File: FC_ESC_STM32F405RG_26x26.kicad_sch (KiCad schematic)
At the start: 211 parts, among them J1 SPI, J12 Conn_02x02_Odd_Even, J14 UART1, J15 UART3_I2C2, J16 MOTOR, J17 MOTOR, J18 MOTOR, J19 MOTOR, J2 Conn_02x04_Odd_Even, J20 USB_A, J21 ESC_PROG, J23 ESC_PROG, J24 ESC_PROG, J25 ESC_PROG, J26 LED_BUZ, J3 ST-LINK, J4 UART4, J7 RC, J8 UART6, J9 OSD, U1 EFM8BB21, U10 FD6288Q, U11 OUTLINE, U12 MPU-6000, U13 BMP280, U15 STM32F405RGTx, U16 RT9013-33GB, U2 EFM8BB21, U3 TPS54560BDDA, U4 FD6288Q, U5 FD6288Q, U6 AT7456, U7 EFM8BB21, U8 EFM8BB21, U9 FD6288Q, Y1 8MHz, Y2 8Mhz

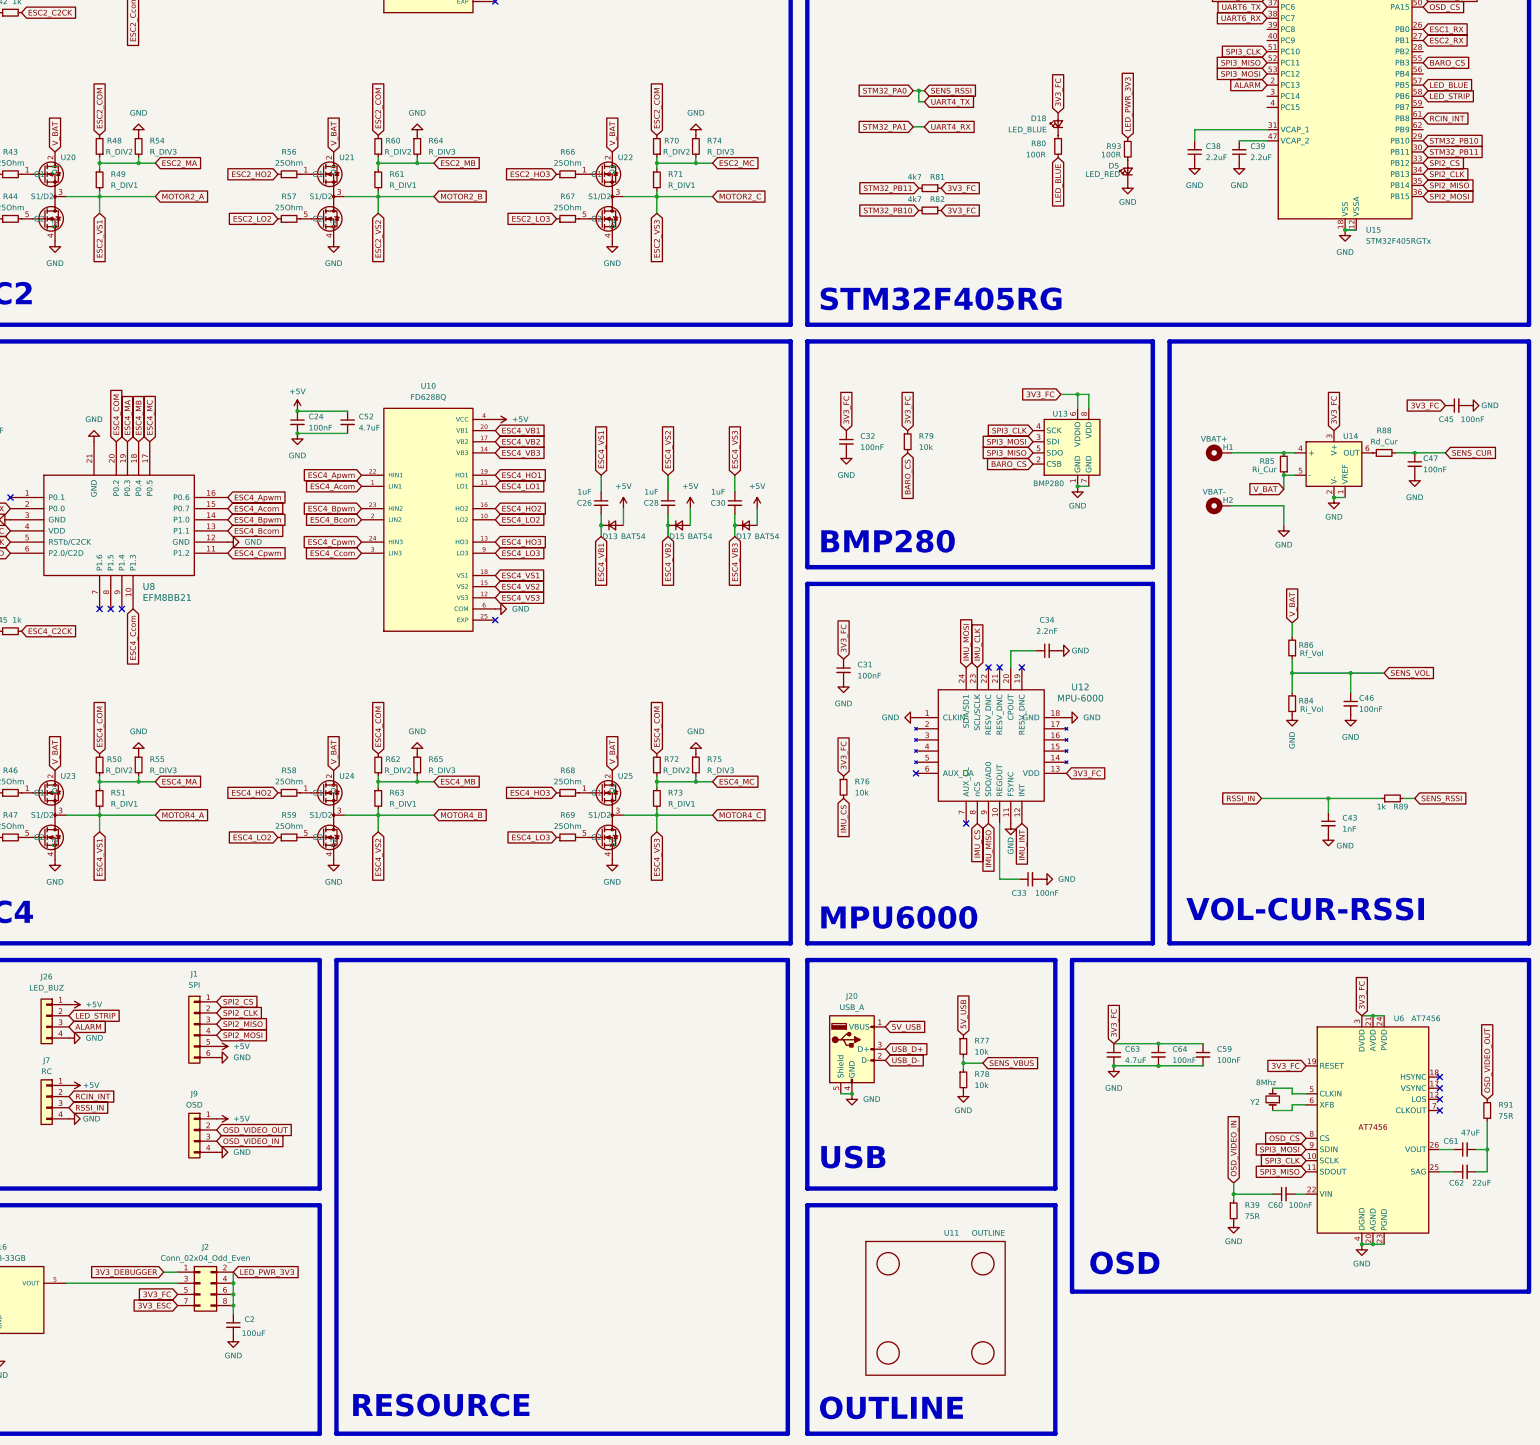
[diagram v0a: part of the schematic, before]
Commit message: update routing
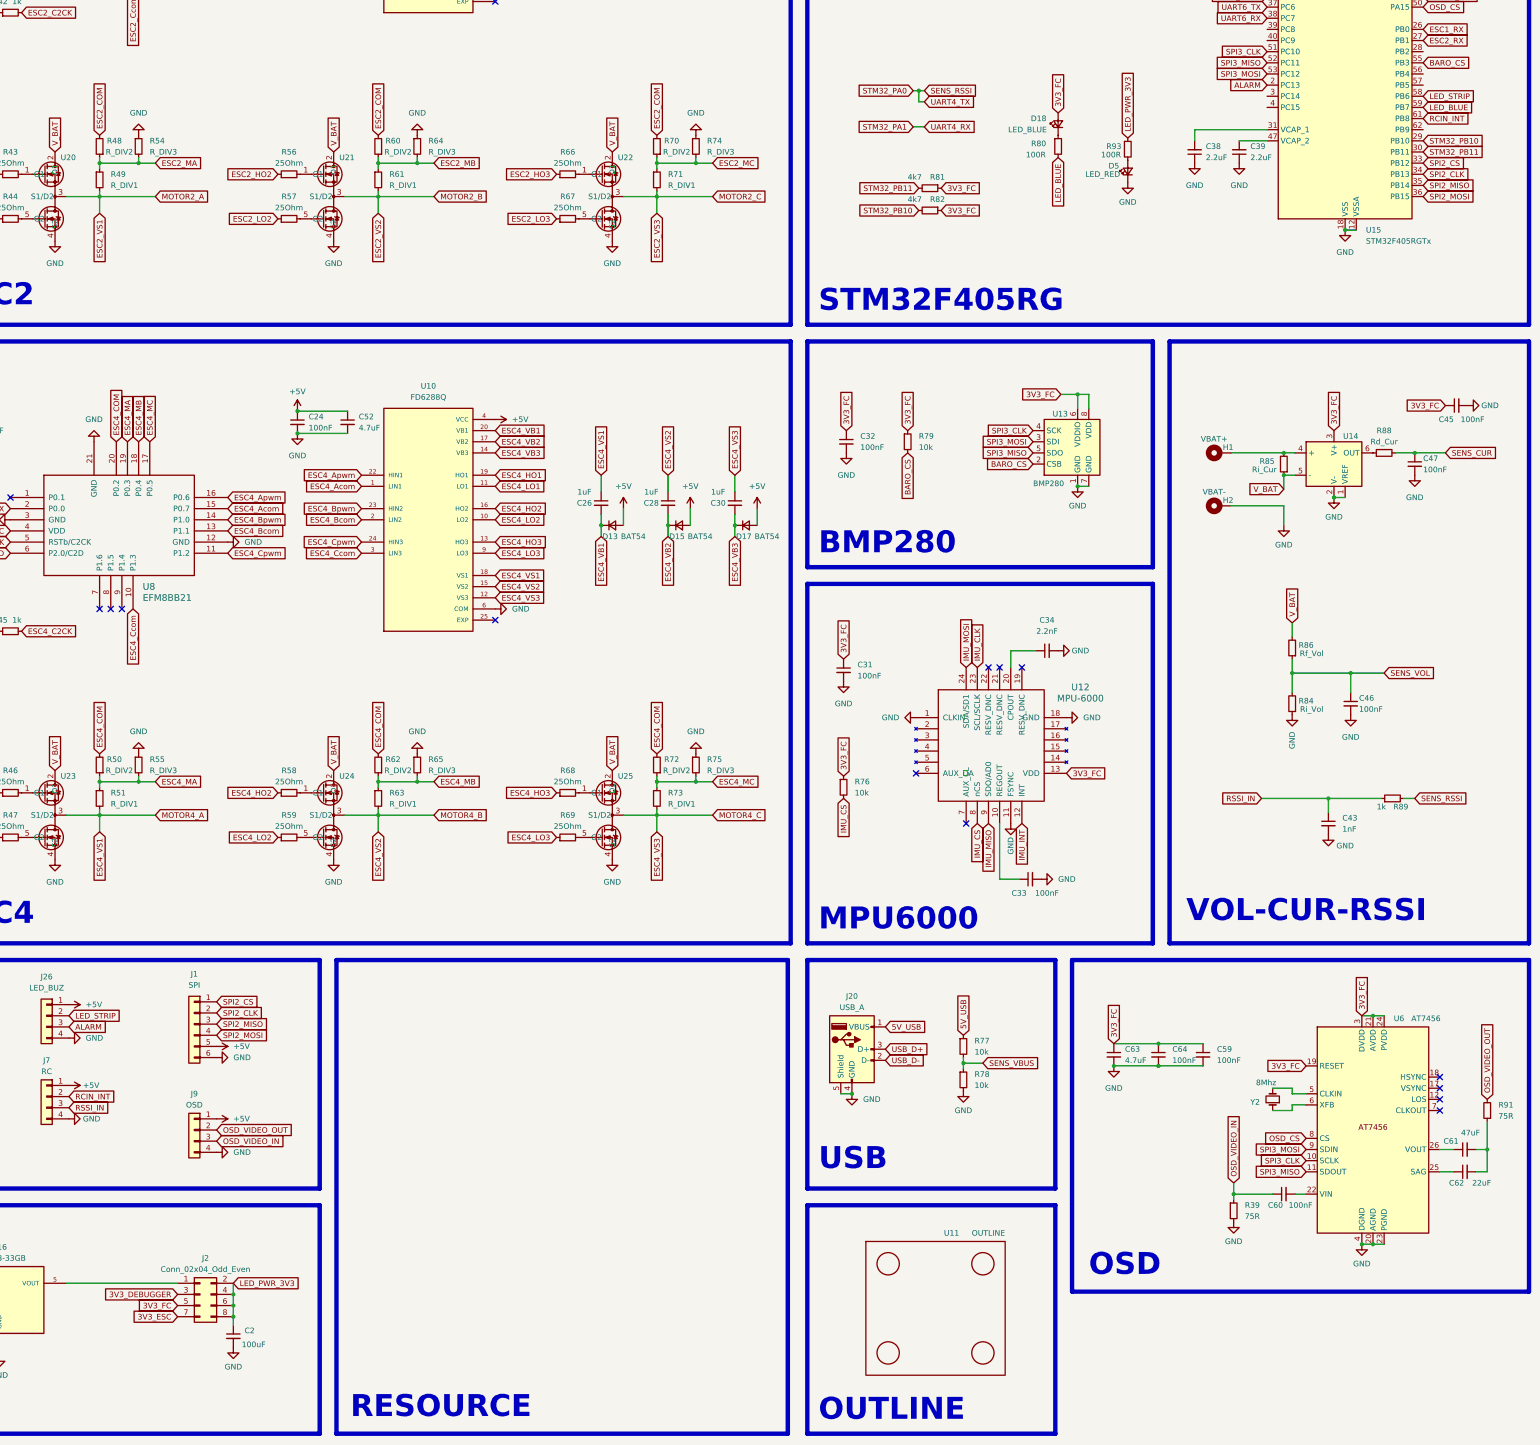
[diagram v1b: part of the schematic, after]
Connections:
- net 3V3_DEBUGGER: now also J2.3 (Pin_3); no longer J2.1 (Pin_1)
- net LED_BLUE: now also U15.59 (PB7); no longer U15.57 (PB5)
- net at U16.5 (VOUT): now also J2.1 (Pin_1); no longer J2.3 (Pin_3)
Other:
- moved on the sheet: C2, J2
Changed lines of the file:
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@@
   (junction (at 180.34 264.16) (diameter 0) (color 0 0 0 0)
   )
-  (junction (at 283.21 375.92) (diameter 0) (color 0 0 0 0)
+  (junction (at 283.21 378.46) (diameter 0) (color 0 0 0 0)
   )
   (junction (at 180.34 115.57) (diameter 0) (color 0 0 0 0)
@@
   (junction (at 388.62 256.54) (diameter 0) (color 0 0 0 0)
   )
-  (junction (at 283.21 373.38) (diameter 0) (color 0 0 0 0)
+  (junction (at 283.21 375.92) (diameter 0) (color 0 0 0 0)
   )
   (junction (at 62.23 115.57) (diameter 0) (color 0 0 0 0)
@@
   (junction (at 98.425 177.165) (diameter 0) (color 0 0 0 0)
   )
-  (junction (at 283.21 370.84) (diameter 0) (color 0 0 0 0)
+  (junction (at 283.21 373.38) (diameter 0) (color 0 0 0 0)
   )
   (junction (at 325.12 115.57) (diameter 0) (color 0 0 0 0)
@@
     (stroke (width 0) (type default))
   )
-  (wire (pts (xy 283.21 368.3) (xy 283.21 370.84))
+  (wire (pts (xy 283.21 370.84) (xy 283.21 373.38))
     (stroke (width 0) (type default))
   )
@@
     (stroke (width 0) (type default))
   )
-  (wire (pts (xy 283.21 373.38) (xy 283.21 375.92))
+  (wire (pts (xy 283.21 375.92) (xy 283.21 378.46))
     (stroke (width 0) (type default))
   )
@@
     (stroke (width 0) (type default))
   )
-  (wire (pts (xy 245.11 370.84) (xy 270.51 370.84))
-    (stroke (width 0) (type default))
-  )
   (wire (pts (xy 53.34 262.89) (xy 53.34 264.16))
     (stroke (width 0) (type default))
@@
     (stroke (width 0) (type default))
   )
-  (wire (pts (xy 283.21 375.92) (xy 283.21 377.825))
+  (wire (pts (xy 283.21 378.46) (xy 283.21 380.365))
     (stroke (width 0) (type default))
   )
@@
     (stroke (width 0) (type default))
   )
-  (wire (pts (xy 270.51 368.3) (xy 267.335 368.3))
+  (wire (pts (xy 245.11 370.84) (xy 270.51 370.84))
     (stroke (width 0) (type default))
   )
@@
     (stroke (width 0) (type default))
   )
-  (wire (pts (xy 283.21 370.84) (xy 283.21 373.38))
+  (wire (pts (xy 283.21 373.38) (xy 283.21 375.92))
     (stroke (width 0) (type default))
   )
@@
     )
   )
-  (global_label "LED_BLUE" (shape input) (at 554.355 97.79 0) (fields_autoplaced)
+  (global_label "LED_BLUE" (shape input) (at 554.355 102.87 0) (fields_autoplaced)
     (effects (font (size 1.27 1.27)) (justify left))
-    (property "Intersheetrefs" "${INTERSHEET_REFS}" (at 566.5325 97.79 0)
+    (property "Intersheetrefs" "${INTERSHEET_REFS}" (at 566.5325 102.87 0)
       (effects (font (size 1.27 1.27)) (justify left) hide)
     )
@@
     )
   )
-  (global_label "3V3_ESC" (shape input) (at 270.51 375.92 180) (fields_autoplaced)
+  (global_label "3V3_ESC" (shape input) (at 270.51 378.46 180) (fields_autoplaced)
     (effects (font (size 1.27 1.27)) (justify right))
-    (property "Intersheetrefs" "${INTERSHEET_REFS}" (at 259.4211 375.92 0)
+    (property "Intersheetrefs" "${INTERSHEET_REFS}" (at 259.4211 378.46 0)
       (effects (font (size 1.27 1.27)) (justify right) hide)
     )
@@
     )
   )
-  (global_label "3V3_FC" (shape input) (at 270.51 373.38 180) (fields_autoplaced)
+  (global_label "3V3_FC" (shape input) (at 270.51 375.92 180) (fields_autoplaced)
     (effects (font (size 1.27 1.27)) (justify right))
-    (property "Intersheetrefs" "${INTERSHEET_REFS}" (at 260.691 373.38 0)
+    (property "Intersheetrefs" "${INTERSHEET_REFS}" (at 260.691 375.92 0)
       (effects (font (size 1.27 1.27)) (justify right) hide)
     )
@@
     )
   )
-  (global_label "LED_PWR_3V3" (shape input) (at 283.21 368.3 0) (fields_autoplaced)
+  (global_label "LED_PWR_3V3" (shape input) (at 283.21 370.84 0) (fields_autoplaced)
     (effects (font (size 1.27 1.27)) (justify left))
-    (property "Intersheetrefs" "${INTERSHEET_REFS}" (at 299.0765 368.3 0)
+    (property "Intersheetrefs" "${INTERSHEET_REFS}" (at 299.0765 370.84 0)
       (effects (font (size 1.27 1.27)) (justify left) hide)
     )
@@
     )
   )
-  (global_label "3V3_DEBUGGER" (shape input) (at 267.335 368.3 180) (fields_autoplaced)
+  (global_label "3V3_DEBUGGER" (shape input) (at 270.51 373.38 180) (fields_autoplaced)
     (effects (font (size 1.27 1.27)) (justify right))
-    (property "Intersheetrefs" "${INTERSHEET_REFS}" (at 249.8961 368.3 0)
+    (property "Intersheetrefs" "${INTERSHEET_REFS}" (at 253.0711 373.38 0)
       (effects (font (size 1.27 1.27)) (justify right) hide)
     )
@@
     )
   )
-  (symbol (lib_id "Connector_Generic:Conn_02x04_Odd_Even") (at 275.59 370.84 0) (unit 1)
+  (symbol (lib_id "Connector_Generic:Conn_02x04_Odd_Even") (at 275.59 373.38 0) (unit 1)
     (in_bom yes) (on_board yes) (dnp no) (fields_autoplaced)
-    (property "Reference" "J2" (at 276.86 362.585 0)
+    (property "Reference" "J2" (at 276.86 365.125 0)
       (effects (font (size 1.27 1.27)))
     )
-    (property "Value" "Conn_02x04_Odd_Even" (at 276.86 365.125 0)
+    (property "Value" "Conn_02x04_Odd_Even" (at 276.86 367.665 0)
       (effects (font (size 1.27 1.27)))
     )
-    (property "Footprint" "Proj_footprint:PinHeader_2x04_P1.27mm_Vertical_SMD" (at 275.59 370.84 0)
+    (property "Footprint" "Proj_footprint:PinHeader_2x04_P1.27mm_Vertical_SMD" (at 275.59 373.38 0)
       (effects (font (size 1.27 1.27)) hide)
     )
-    (property "Datasheet" "~" (at 275.59 370.84 0)
+    (property "Datasheet" "~" (at 275.59 373.38 0)
       (effects (font (size 1.27 1.27)) hide)
     )
@@
     )
   )
-  (symbol (lib_id "Device:C_Small") (at 283.21 380.365 0) (unit 1)
+  (symbol (lib_id "Device:C_Small") (at 283.21 382.905 0) (unit 1)
     (in_bom yes) (on_board yes) (dnp no)
-    (property "Reference" "C2" (at 285.75 379.095 0)
+    (property "Reference" "C2" (at 285.75 381.635 0)
       (effects (font (size 1.27 1.27)) (justify left))
     )
-    (property "Value" "100uF" (at 285.115 382.27 0)
+    (property "Value" "100uF" (at 285.115 384.81 0)
       (effects (font (size 1.27 1.27)) (justify left))
     )
-    (property "Footprint" "Capacitor_SMD:C_1210_3225Metric_Pad1.33x2.70mm_HandSolder" (at 283.21 380.365 0)
+    (property "Footprint" "Capacitor_SMD:C_1210_3225Metric_Pad1.33x2.70mm_HandSolder" (at 283.21 382.905 0)
       (effects (font (size 1.27 1.27)) hide)
     )
-    (property "Datasheet" "~" (at 283.21 380.365 0)
+    (property "Datasheet" "~" (at 283.21 382.905 0)
       (effects (font (size 1.27 1.27)) hide)
     )
@@
     )
   )
-  (symbol (lib_id "power:GND") (at 283.21 382.905 0) (unit 1)
+  (symbol (lib_id "power:GND") (at 283.21 385.445 0) (unit 1)
     (in_bom yes) (on_board yes) (dnp no) (fields_autoplaced)
-    (property "Reference" "#PWR03" (at 283.21 389.255 0)
+    (property "Reference" "#PWR03" (at 283.21 391.795 0)
       (effects (font (size 1.27 1.27)) hide)
     )
-    (property "Value" "GND" (at 283.21 387.35 0)
+    (property "Value" "GND" (at 283.21 389.89 0)
       (effects (font (size 1.27 1.27)))
     )
-    (property "Footprint" "" (at 283.21 382.905 0)
+    (property "Footprint" "" (at 283.21 385.445 0)
       (effects (font (size 1.27 1.27)) hide)
     )
-    (property "Datasheet" "" (at 283.21 382.905 0)
+    (property "Datasheet" "" (at 283.21 385.445 0)
       (effects (font (size 1.27 1.27)) hide)
     )
